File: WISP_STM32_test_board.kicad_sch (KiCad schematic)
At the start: 37 parts, among them J1 Conn_02x05_Odd_Even, J2 Conn_02x01, J3 Conn_02x01, J4 Conn_01x10_Pin, J5 Conn_01x02_Pin, SW1 SW_Push, SW2 SW_Push, SW5 SW_SPST, U1 MAX3072E, U2 MAX3072E, U4 STM32F446RETx, U6 AP63203WU

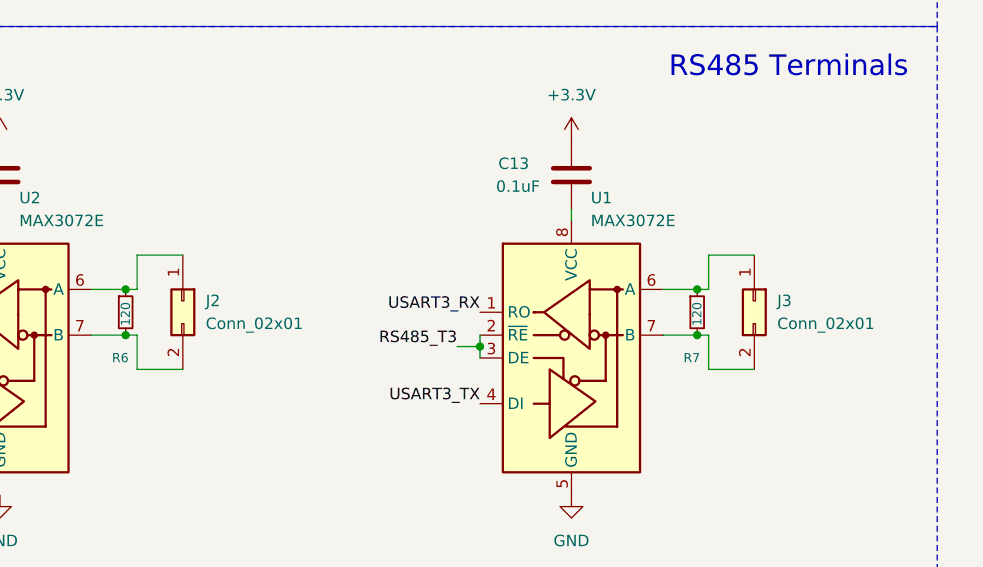
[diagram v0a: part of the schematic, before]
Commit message: John revisions 9/7
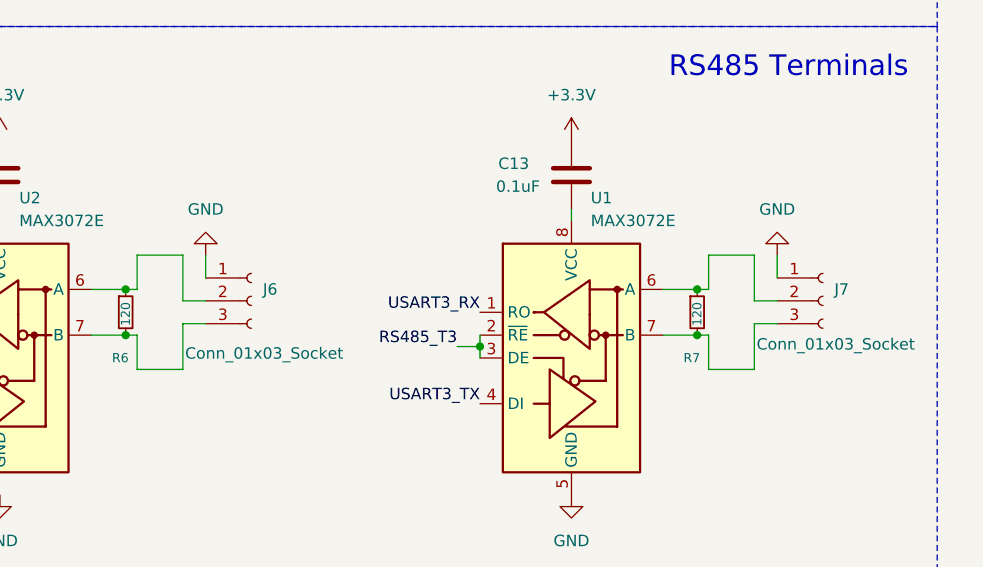
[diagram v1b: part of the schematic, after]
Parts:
- removed J2, J3: Conn_02x01, TerminalBlock:TerminalBlock_Xinya_XY308-2.54-2P_1x02_P2.54mm_Horizontal, symbol Connector_Generic:Conn_02x01
- added J6, J7: Conn_01x03_Socket, TerminalBlock:TerminalBlock_Xinya_XY308-2.54-3P_1x03_P2.54mm_Horizontal, symbol Connector:Conn_01x03_Socket
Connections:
- net GND: now also J6.1 (Pin_1), J7.1 (Pin_1)
- net at R6.1, U2.6 (A): now also J6.2 (Pin_2)
- net at R6.2, U2.7 (B): now also J6.3 (Pin_3)
- net at R7.1, U1.6 (A): now also J7.2 (Pin_2)
- net at R7.2, U1.7 (B): now also J7.3 (Pin_3)
